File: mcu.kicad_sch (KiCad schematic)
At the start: 25 parts, among them U1 W25Q32JVSS, U2 RP2040, Y1 12M 18pF

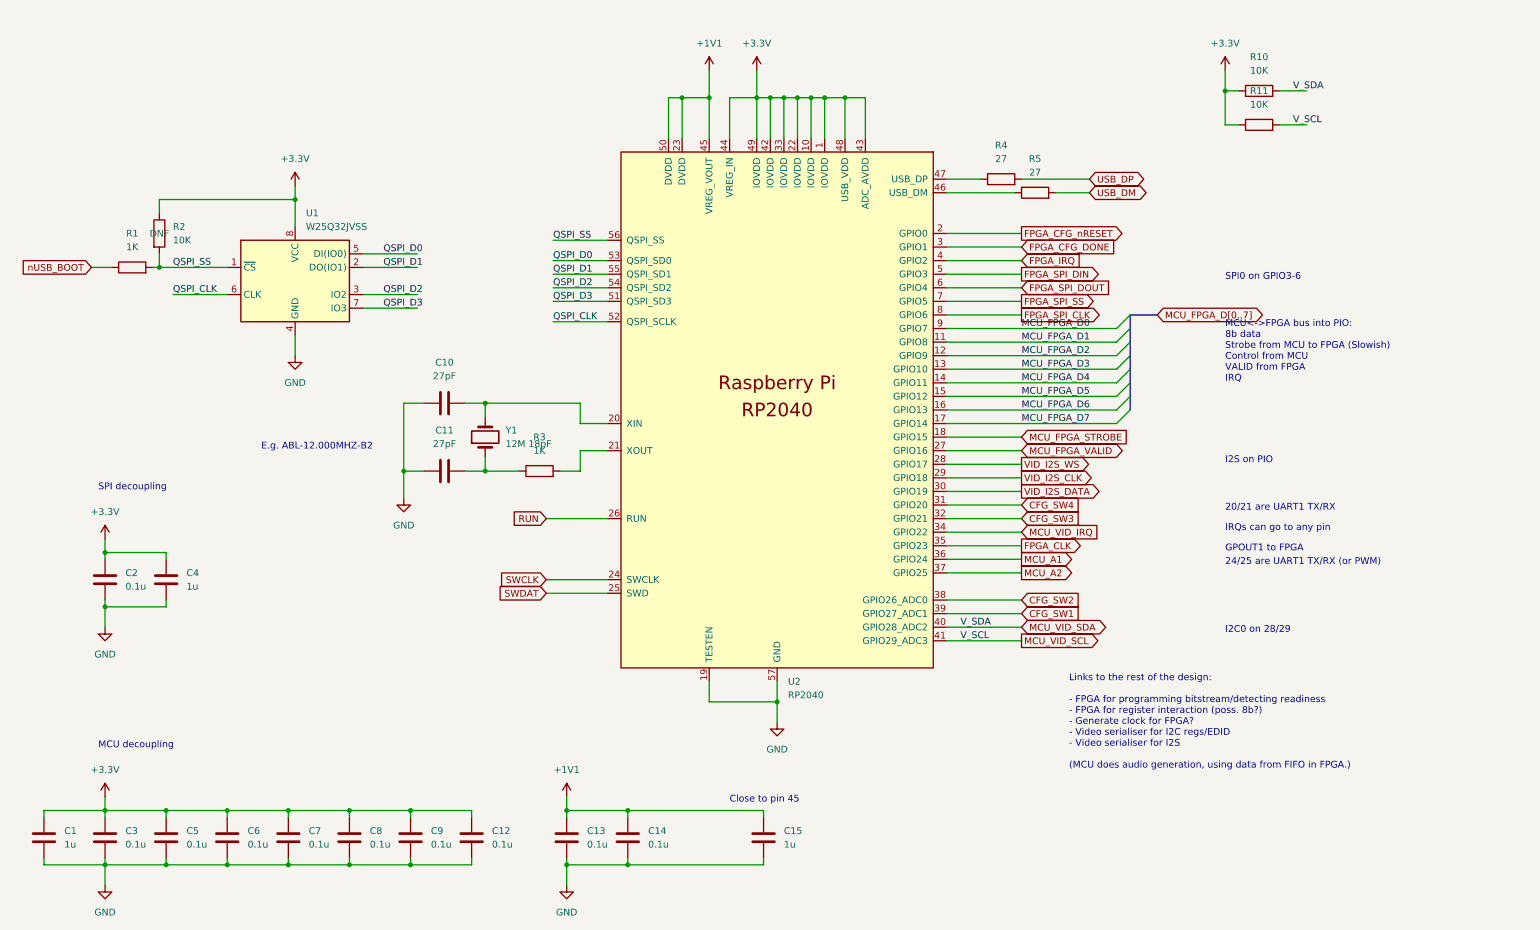
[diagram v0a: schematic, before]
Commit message: v2: ADV7513 and FFC
Large work much progress - almost routed
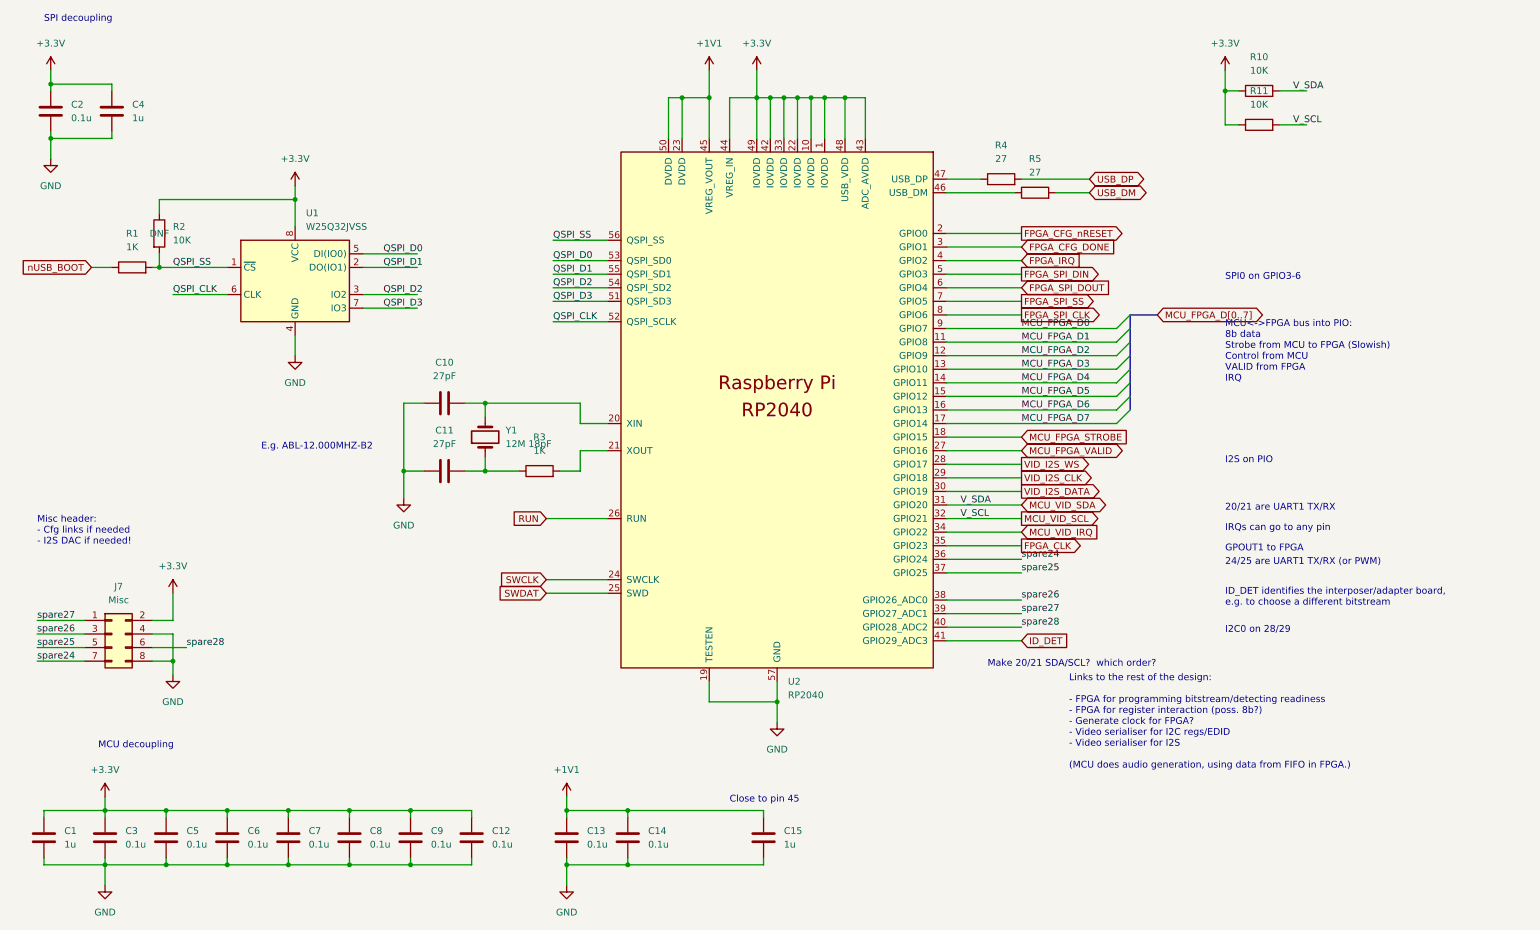
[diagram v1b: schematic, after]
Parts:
- added J7: Misc, Connector_PinHeader_2.00mm:PinHeader_2x04_P2.00mm_Vertical, symbol Connector_Generic:Conn_02x04_Odd_Even
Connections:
- net CFG_SW3 is gone; now on net MCU_VID_SCL: U2.32 (GPIO21)
- net CFG_SW4 is gone; now on net MCU_VID_SDA: U2.31 (GPIO20)
- net +3V3: now also J7.2 (Pin_2)
- net GND: now also J7.4 (Pin_4), J7.8 (Pin_8)
- net MCU_VID_SCL: no longer U2.41 (GPIO29_ADC3)
- net MCU_VID_SDA: no longer U2.40 (GPIO28_ADC2)
- net CFG_SW1 renamed spare27
- net spare27: now also J7.1 (Pin_1)
- net CFG_SW2 renamed spare26
- net spare26: now also J7.3 (Pin_3)
- net MCU_A1 renamed spare24
- net spare24: now also J7.7 (Pin_7)
- net MCU_A2 renamed spare25
- net spare25: now also J7.5 (Pin_5)
- new net ID_DET: U2.41 (GPIO29_ADC3)
- new net spare28: J7.6 (Pin_6), U2.40 (GPIO28_ADC2)
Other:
- note added: "ID_DET identifies the interposer/adapter board, e.g. to choose a different bitstream"
- note added: "Make 20/21 SDA/SCL? which order?"
- note added: "Misc header: - Cfg links if needed - I2S DAC if needed!"
- moved on the sheet: C2, C4
